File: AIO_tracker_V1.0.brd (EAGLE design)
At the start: 47 x 90 mm, 76 parts, among them J1 EDGE_ICSP, Q1 MOSFET-PCHANNELSMD, U2 USD-SOCKETNEW, X1 SMA-142-0701-881/886, Y1 ABRACON_ABM3_CRYSTAL

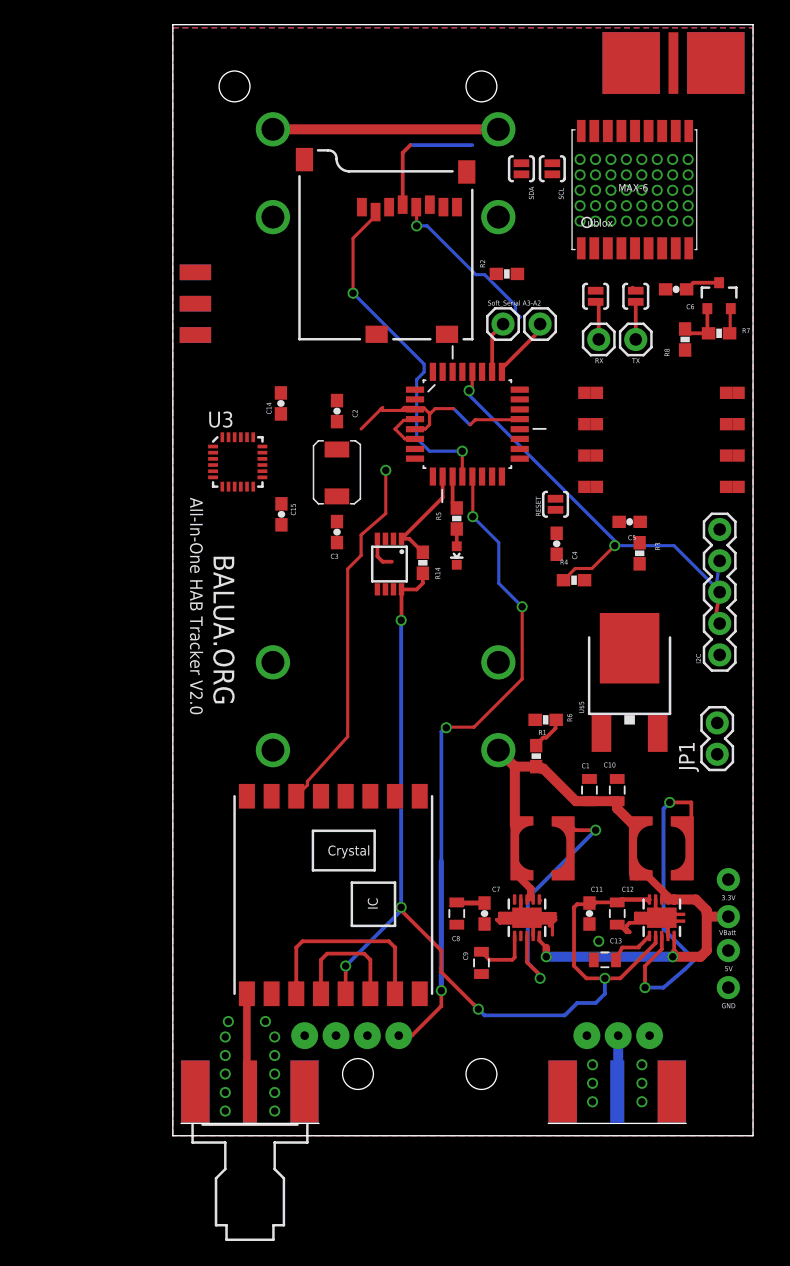
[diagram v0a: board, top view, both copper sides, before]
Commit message: size and placement defined
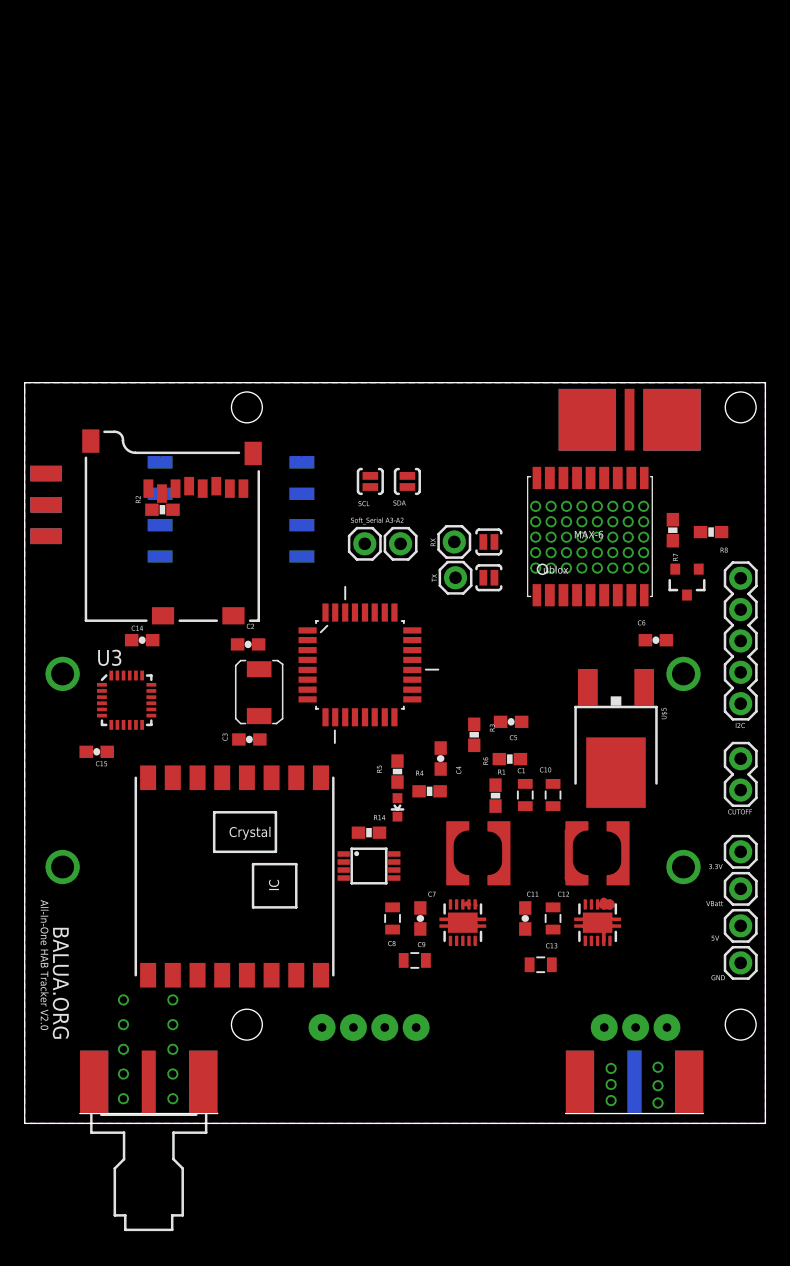
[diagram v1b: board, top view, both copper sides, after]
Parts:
- removed JP1: M02PTH, SparkFun-Connectors:1X02
- removed SJ2: SOLDERJUMPERNO, SparkFun-Passives:SJ_2S-NO
- added CUTOFF: M02PTH, SparkFun-Connectors:1X02
- 3.3V, 5V, GND, VBATT: value M01SMDNS -> M01PTH; device SparkFun-Connectors:1X01NS -> SparkFun-Connectors:1X01
- U$3: value RADIOMETRIX-HX1 -> NTX2-VERTICAL; device Ava:RADIOMETRIX-HX1 -> Ava:NTX2-VERTICAL
- moved TP12 49.2 mm to (-2.53, 29.9), flipped to the bottom, turned to 180 degrees
- moved TP16 48.1 mm to (-2.53, 32.5), flipped to the bottom, turned to 180 degrees
- moved TP9 47.5 mm to (-2.53, 35.0), flipped to the bottom, turned to 180 degrees
- moved TP13 47.4 mm to (-2.53, 37.5), flipped to the bottom, turned to 180 degrees
- moved TP11 47.2 mm to (-1.51, 29.9), flipped to the bottom, turned to 180 degrees
- moved TP15 46.1 mm to (-1.51, 32.5), flipped to the bottom, turned to 180 degrees
- moved TP10 45.4 mm to (-1.51, 35.0), flipped to the bottom, turned to 180 degrees
- moved TP14 45.4 mm to (-1.51, 37.5), flipped to the bottom, turned to 180 degrees
- moved BAT1 36.1 mm to (15.2, 4.77), turned to 0 degrees
- moved R2 33.8 mm to (-1.84, 33.7)
- moved SJ3 29.3 mm to (15.0, 36.0)
- moved U$2 29.1 mm to (36.0, 41.0)
- moved U2 28.6 mm to (5.96, 24.7)
- moved C6 28.5 mm to (38.1, 23.1), turned to 0 degrees
- moved U$1 28.3 mm to (32.9, 31.7)
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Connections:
- removed net N$8: C4.1, SJ2.1
- net 3.3V: now also C4.1; no longer SJ2.2
- net CUTOUT: now also CUTOFF.2; no longer JP1.2
- net GND: now also CUTOFF.1, U$3.RFGND1; no longer JP1.1, U$3.RFGND
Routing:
- net 3.3V: track 106.4 -> 0.00 mm, vias 5 -> 0
- net 5VEN: track 54.0 -> 0.00 mm, vias 4 -> 0
- net VBATT: track 59.8 -> 7.33 mm, vias 2 -> 0
- net GND: track 53.7 -> 1.41 mm, vias 59 -> 56
- net SCL: track 36.5 -> 0.00 mm, vias 2 -> 0
- net RFM22_NIRQ: track 29.5 -> 0.00 mm, vias 1 -> 0
- net SD_CS: track 27.9 -> 0.00 mm, vias 2 -> 0
- net N$19: track 27.9 -> 0.00 mm, vias 2 -> 0
- net N$7: track 20.8 -> 0.00 mm, vias 2 -> 0
- net N$10: track 18.3 -> 0.00 mm
- net N$29: track 16.8 -> 0.00 mm
- net SCK: track 13.3 -> 0.00 mm, vias 1 -> 0
- net N$30: track 10.3 -> 0.00 mm
- net TEMP: track 8.60 -> 0.00 mm
- net N$13: track 8.18 -> 0.00 mm
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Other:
- board size 47 x 90 mm -> 60 x 60 mm
- board text removed: "RESET"
